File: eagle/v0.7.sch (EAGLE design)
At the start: 19 parts

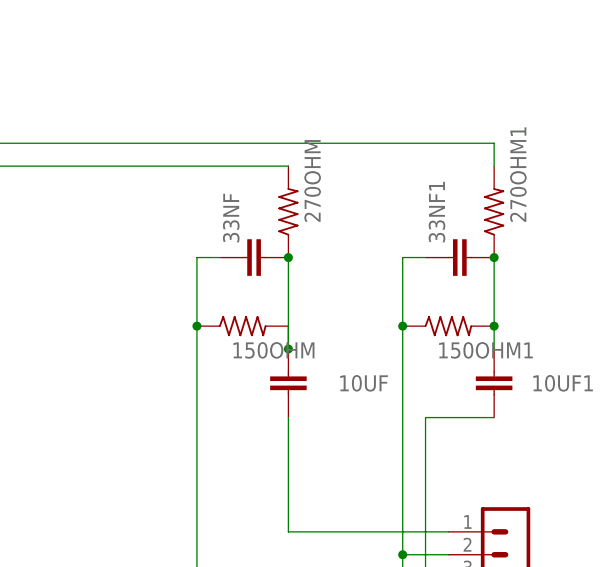
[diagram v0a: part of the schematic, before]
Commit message: Board version v0.7
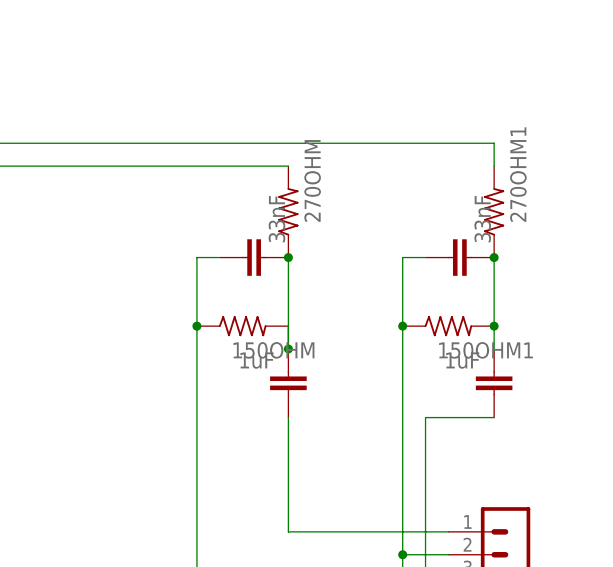
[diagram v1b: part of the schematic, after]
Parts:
- removed 33NF, 33NF1: (no value), rcl:C-EU025-025X050
- added C1, C2: 33nF, capacitor-wima:C5/5
- E1, E2: value (none) -> 1uF
- renumbered 10UF to E1, 10UF1 to E2
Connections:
- net GND: now also C1.1, C2.1; no longer 33NF.1, 33NF1.1
- net N$1: now also C1.2; no longer 33NF.2
- net N$7: now also C2.2; no longer 33NF1.2
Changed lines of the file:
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@@
 <part name="RFID" library="con-lstb" library_urn="urn:adsk.eagle:library:162" deviceset="MA08-1" device="" package3d_urn="urn:adsk.eagle:package:8343/1"/>
 <part name="LCD" library="con-lstb" library_urn="urn:adsk.eagle:library:162" deviceset="MA09-1" device="" package3d_urn="urn:adsk.eagle:package:8350/1"/>
-<part name="33NF" library="rcl" library_urn="urn:adsk.eagle:library:334" deviceset="C-EU" device="025-025X050" package3d_urn="urn:adsk.eagle:package:23629/2"/>
 <part name="LIPO" library="con-3m" library_urn="urn:adsk.eagle:library:119" deviceset="2514-" device="" package3d_urn="urn:adsk.eagle:package:5575/1"/>
 <part name="LED1" library="led" library_urn="urn:adsk.eagle:library:259" deviceset="LED" device="3MM" package3d_urn="urn:adsk.eagle:package:15797/1"/>
@@
 <part name="270OHM" library="rcl" library_urn="urn:adsk.eagle:library:334" deviceset="R-US_" device="0204/5" package3d_urn="urn:adsk.eagle:package:23488/1"/>
 <part name="150OHM" library="rcl" library_urn="urn:adsk.eagle:library:334" deviceset="R-US_" device="0204/5" package3d_urn="urn:adsk.eagle:package:23488/1"/>
-<part name="10UF" library="rcl" library_urn="urn:adsk.eagle:library:334" deviceset="C-EU" device="025-025X050" package3d_urn="urn:adsk.eagle:package:23629/2"/>
+<part name="E1" library="rcl" library_urn="urn:adsk.eagle:library:334" deviceset="C-EU" device="025-025X050" package3d_urn="urn:adsk.eagle:package:23629/2" value="1uF"/>
 <part name="RLED2" library="rcl" library_urn="urn:adsk.eagle:library:334" deviceset="R-US_" device="0204/5" package3d_urn="urn:adsk.eagle:package:23488/1"/>
 <part name="LED2" library="led" library_urn="urn:adsk.eagle:library:259" deviceset="LED" device="3MM" package3d_urn="urn:adsk.eagle:package:15797/1"/>
@@
 <part name="LED3" library="led" library_urn="urn:adsk.eagle:library:259" deviceset="LED" device="3MM" package3d_urn="urn:adsk.eagle:package:15797/1"/>
 <part name="AUDIOOUT" library="con-lstb" library_urn="urn:adsk.eagle:library:162" deviceset="MA03-1" device="" package3d_urn="urn:adsk.eagle:package:8339/1"/>
-<part name="33NF1" library="rcl" library_urn="urn:adsk.eagle:library:334" deviceset="C-EU" device="025-025X050" package3d_urn="urn:adsk.eagle:package:23629/2"/>
 <part name="270OHM1" library="rcl" library_urn="urn:adsk.eagle:library:334" deviceset="R-US_" device="0204/5" package3d_urn="urn:adsk.eagle:package:23488/1"/>
 <part name="150OHM1" library="rcl" library_urn="urn:adsk.eagle:library:334" deviceset="R-US_" device="0204/5" package3d_urn="urn:adsk.eagle:package:23488/1"/>
-<part name="10UF1" library="rcl" library_urn="urn:adsk.eagle:library:334" deviceset="C-EU" device="025-025X050" package3d_urn="urn:adsk.eagle:package:23629/2"/>
+<part name="E2" library="rcl" library_urn="urn:adsk.eagle:library:334" deviceset="C-EU" device="025-025X050" package3d_urn="urn:adsk.eagle:package:23629/2" value="1uF"/>
+<part name="C1" library="capacitor-wima" library_urn="urn:adsk.eagle:library:116" deviceset="C" device="5/5" package3d_urn="urn:adsk.eagle:package:5428/1" value="33nF"/>
+<part name="C2" library="capacitor-wima" library_urn="urn:adsk.eagle:library:116" deviceset="C" device="5/5" package3d_urn="urn:adsk.eagle:package:5428/1" value="33nF"/>
 </parts>
 <sheets>
@@
 <attribute name="NAME" x="97.79" y="29.718" size="1.778" layer="95" rot="R180"/>
 </instance>
-<instance part="33NF" gate="G$1" x="167.64" y="53.34" smashed="yes" rot="R90">
-<attribute name="NAME" x="167.259" y="54.864" size="1.778" layer="95" rot="R90"/>
-<attribute name="VALUE" x="172.339" y="54.864" size="1.778" layer="96" rot="R90"/>
-</instance>
 <instance part="LIPO" gate="-1" x="-35.56" y="93.98" smashed="yes">
 <attribute name="NAME" x="-36.83" y="94.869" size="1.778" layer="95" rot="R180"/>
@@
 <attribute name="VALUE" x="163.83" y="42.418" size="1.778" layer="96"/>
 </instance>
-<instance part="10UF" gate="G$1" x="172.72" y="38.1" smashed="yes" rot="R180">
-<attribute name="NAME" x="183.896" y="40.259" size="1.778" layer="95" rot="R180"/>
+<instance part="E1" gate="G$1" x="172.72" y="38.1" smashed="yes" rot="R180">
 <attribute name="VALUE" x="171.196" y="42.799" size="1.778" layer="96" rot="R180"/>
 </instance>
@@
 <attribute name="NAME" x="199.39" y="14.478" size="1.778" layer="95" rot="R180"/>
 </instance>
-<instance part="33NF1" gate="G$1" x="190.5" y="53.34" smashed="yes" rot="R90">
-<attribute name="NAME" x="190.119" y="54.864" size="1.778" layer="95" rot="R90"/>
-<attribute name="VALUE" x="195.199" y="54.864" size="1.778" layer="96" rot="R90"/>
-</instance>
 <instance part="270OHM1" gate="G$1" x="195.58" y="58.42" smashed="yes" rot="R90">
 <attribute name="NAME" x="199.1614" y="57.15" size="1.778" layer="95" rot="R90"/>
@@
 <attribute name="VALUE" x="186.69" y="42.418" size="1.778" layer="96"/>
 </instance>
-<instance part="10UF1" gate="G$1" x="195.58" y="38.1" smashed="yes" rot="R180">
-<attribute name="NAME" x="206.756" y="40.259" size="1.778" layer="95" rot="R180"/>
+<instance part="E2" gate="G$1" x="195.58" y="38.1" smashed="yes" rot="R180">
 <attribute name="VALUE" x="194.056" y="42.799" size="1.778" layer="96" rot="R180"/>
+</instance>
+<instance part="C1" gate="G$1" x="167.64" y="53.34" smashed="yes" rot="R90">
+<attribute name="VALUE" x="172.339" y="54.864" size="1.778" layer="96" rot="R90"/>
+</instance>
+<instance part="C2" gate="G$1" x="190.5" y="53.34" smashed="yes" rot="R90">
+<attribute name="VALUE" x="195.199" y="54.864" size="1.778" layer="96" rot="R90"/>
 </instance>
 </instances>
@@
 <segment>
 <pinref part="270OHM" gate="G$1" pin="1"/>
-<pinref part="33NF" gate="G$1" pin="2"/>
 <pinref part="150OHM" gate="G$1" pin="2"/>
-<pinref part="10UF" gate="G$1" pin="2"/>
+<pinref part="E1" gate="G$1" pin="2"/>
 <wire x1="172.72" y1="53.34" x2="172.72" y2="43.18" width="0.1524" layer="91"/>
-<junction x="172.72" y="53.34"/>
 <junction x="172.72" y="43.18"/>
 <wire x1="172.72" y1="43.18" x2="172.72" y2="45.72" width="0.1524" layer="91"/>
+<pinref part="C1" gate="G$1" pin="2"/>
+<junction x="172.72" y="53.34"/>
 </segment>
 </net>
@@
 <junction x="101.6" y="-2.54"/>
 <wire x1="101.6" y1="-2.54" x2="124.46" y2="-2.54" width="0.1524" layer="91"/>
-<pinref part="33NF" gate="G$1" pin="1"/>
 <wire x1="124.46" y1="-2.54" x2="147.32" y2="-2.54" width="0.1524" layer="91"/>
 <wire x1="147.32" y1="-2.54" x2="162.56" y2="-2.54" width="0.1524" layer="91"/>
@@
 <pinref part="LED3" gate="G$1" pin="C"/>
 <junction x="147.32" y="-2.54"/>
-<pinref part="33NF1" gate="G$1" pin="1"/>
 <wire x1="187.96" y1="53.34" x2="185.42" y2="53.34" width="0.1524" layer="91"/>
 <pinref part="150OHM1" gate="G$1" pin="1"/>
@@
 <wire x1="190.5" y1="20.32" x2="185.42" y2="20.32" width="0.1524" layer="91"/>
 <junction x="185.42" y="20.32"/>
+<pinref part="C1" gate="G$1" pin="1"/>
+<pinref part="C2" gate="G$1" pin="1"/>
 </segment>
 </net>
@@
 <net name="N$7" class="0">
 <segment>
-<pinref part="33NF1" gate="G$1" pin="2"/>
 <pinref part="270OHM1" gate="G$1" pin="1"/>
 <pinref part="150OHM1" gate="G$1" pin="2"/>
-<pinref part="10UF1" gate="G$1" pin="2"/>
+<pinref part="E2" gate="G$1" pin="2"/>
 <wire x1="195.58" y1="43.18" x2="195.58" y2="45.72" width="0.1524" layer="91"/>
 <wire x1="195.58" y1="53.34" x2="195.58" y2="45.72" width="0.1524" layer="91"/>
+<junction x="195.58" y="45.72"/>
+<pinref part="C2" gate="G$1" pin="2"/>
 <junction x="195.58" y="53.34"/>
-<junction x="195.58" y="45.72"/>
 </segment>
 </net>
@@
 <pinref part="AUDIOOUT" gate="G$1" pin="1"/>
 <wire x1="190.5" y1="22.86" x2="172.72" y2="22.86" width="0.1524" layer="91"/>
-<pinref part="10UF" gate="G$1" pin="1"/>
+<pinref part="E1" gate="G$1" pin="1"/>
 <wire x1="172.72" y1="22.86" x2="172.72" y2="35.56" width="0.1524" layer="91"/>
 </segment>
@@
 <wire x1="190.5" y1="17.78" x2="187.96" y2="17.78" width="0.1524" layer="91"/>
 <wire x1="187.96" y1="17.78" x2="187.96" y2="35.56" width="0.1524" layer="91"/>
-<pinref part="10UF1" gate="G$1" pin="1"/>
+<pinref part="E2" gate="G$1" pin="1"/>
 <wire x1="187.96" y1="35.56" x2="195.58" y2="35.56" width="0.1524" layer="91"/>
 </segment>
